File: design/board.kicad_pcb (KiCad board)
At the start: 2 copper layers, 123.4 x 53.2 mm, 37 parts, among them J1 Conn_02x04_Odd_Even, SW1 SW_Push, SW2 SW_Push, SW3 SW_Push, SW4 SW_Push, SW5 SW_Push, SW6 SW_Push, U1 LM555, U2 LM555, U3 LM555, U4 LM555, U5 LM555, U6 LM555

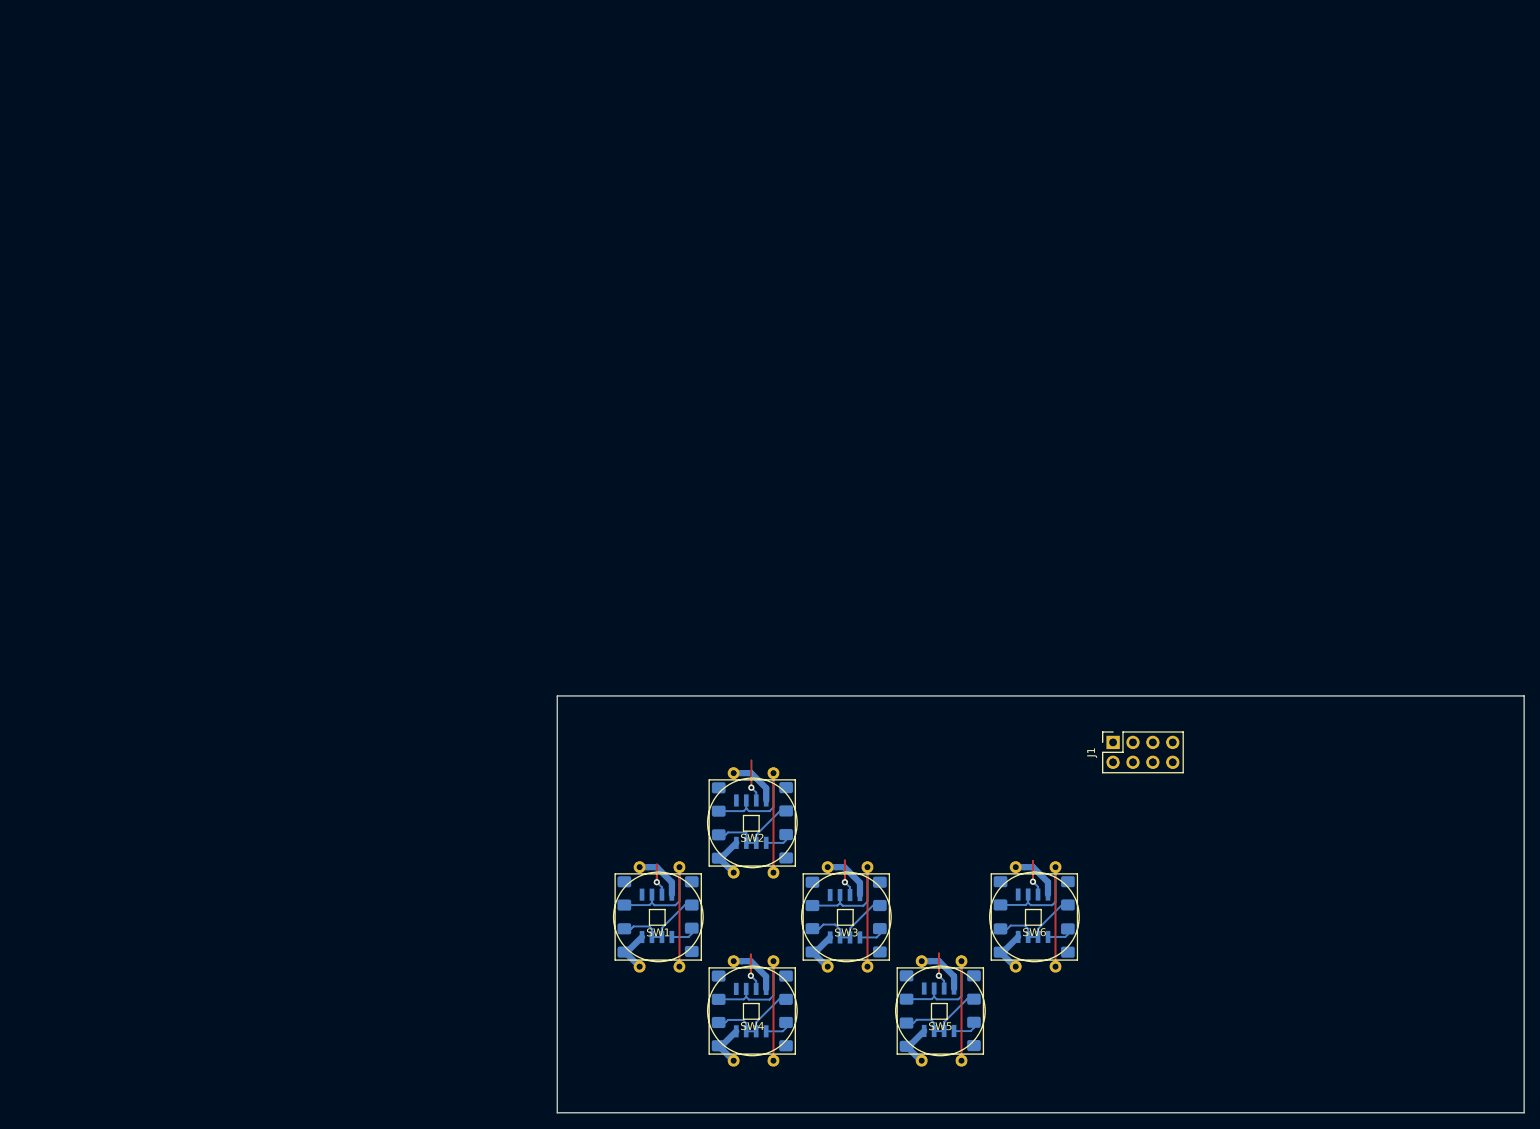
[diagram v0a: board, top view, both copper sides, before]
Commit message: v1 of the controller done.
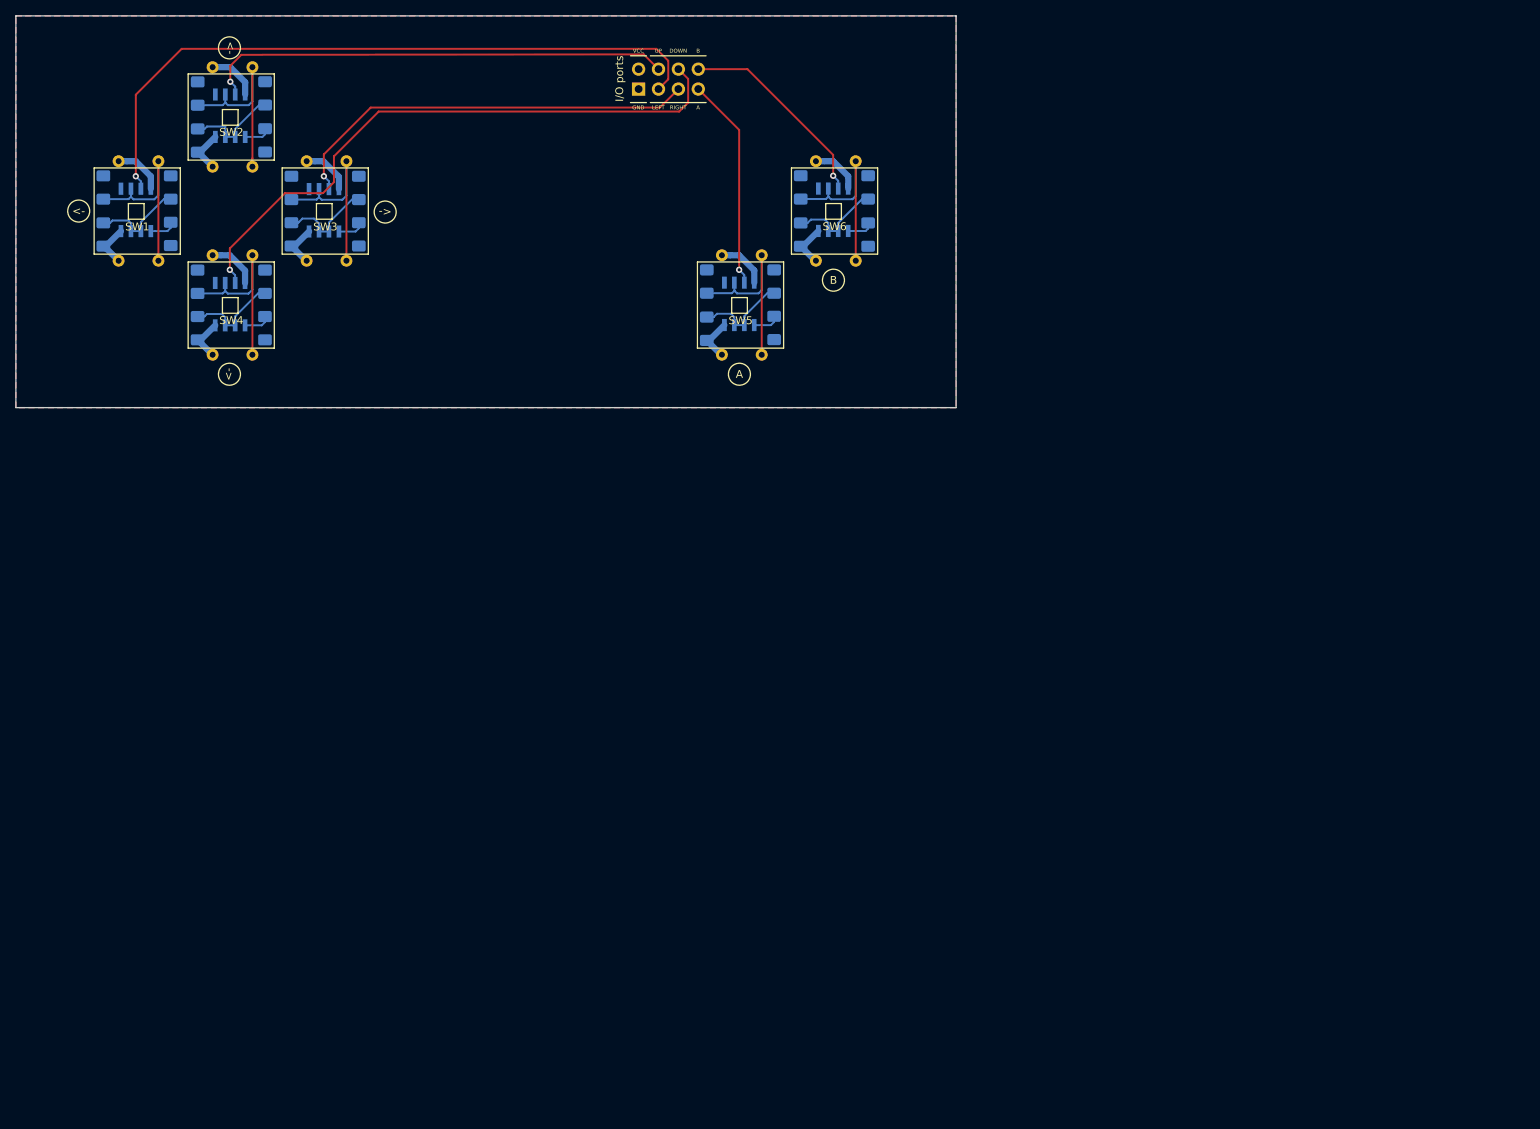
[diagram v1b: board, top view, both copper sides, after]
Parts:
- J1: moved to B.Cu
- moved C7 112.0 mm to (52.8, 56.9)
- moved R8 112.0 mm to (44.2, 56.9)
- moved SW1 112.0 mm to (36.3, 41.6)
- moved SW3 112.0 mm to (60.3, 41.6)
- moved SW4 112.0 mm to (48.3, 53.6)
- moved U4 112.0 mm to (48.3, 53.6)
- moved C1 112.0 mm to (40.8, 44.8)
- moved C2 112.0 mm to (40.8, 38.9)
- moved C3 112.0 mm to (52.8, 32.9)
- moved C4 112.0 mm to (52.8, 26.9)
- moved C5 112.0 mm to (64.8, 44.9)
- moved C6 112.0 mm to (64.8, 39.0)
- moved C8 112.0 mm to (52.8, 50.9)
- moved R1 112.0 mm to (32.2, 38.9)
- moved R2 112.0 mm to (32.2, 44.9)
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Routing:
- net /L_out: track 4.14 -> 87.4 mm
- net /D_out: track 4.69 -> 77.6 mm
- net /U_out: track 5.83 -> 60.4 mm
- net /R_out: track 4.71 -> 53.4 mm
- net /A_out: track 4.78 -> 27.2 mm
- net /B_out: track 4.57 -> 26.3 mm
- added copper zone on B.Cu, net /GND
- added copper zone on F.Cu, net /VCC
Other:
- board size 123.4 x 53.2 mm -> 120 x 50 mm
- board text added: "<-"
- board text added: "A"
- board text added: "B"
- board text added: "DOWN"
- board text added: "GND"
- board text added: "I/O ports"
- board text added: "LEFT"
- board text added: "RIGHT"
- board text added: "UP"
- board text added: "VCC"
